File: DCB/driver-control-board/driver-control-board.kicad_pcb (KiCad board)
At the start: 2 copper layers, 92.7 x 59.2 mm, 33 parts, among them J1 Conn_01x05, J2 Conn_01x14, J3 Conn_01x08, J4 Conn_01x23, U1 STM32F413CGUx, U2 LD1117S33TR_SOT223, U3 R-78B5.0-2.0, U4 MCP2551-I-SN, Y1 Crystal

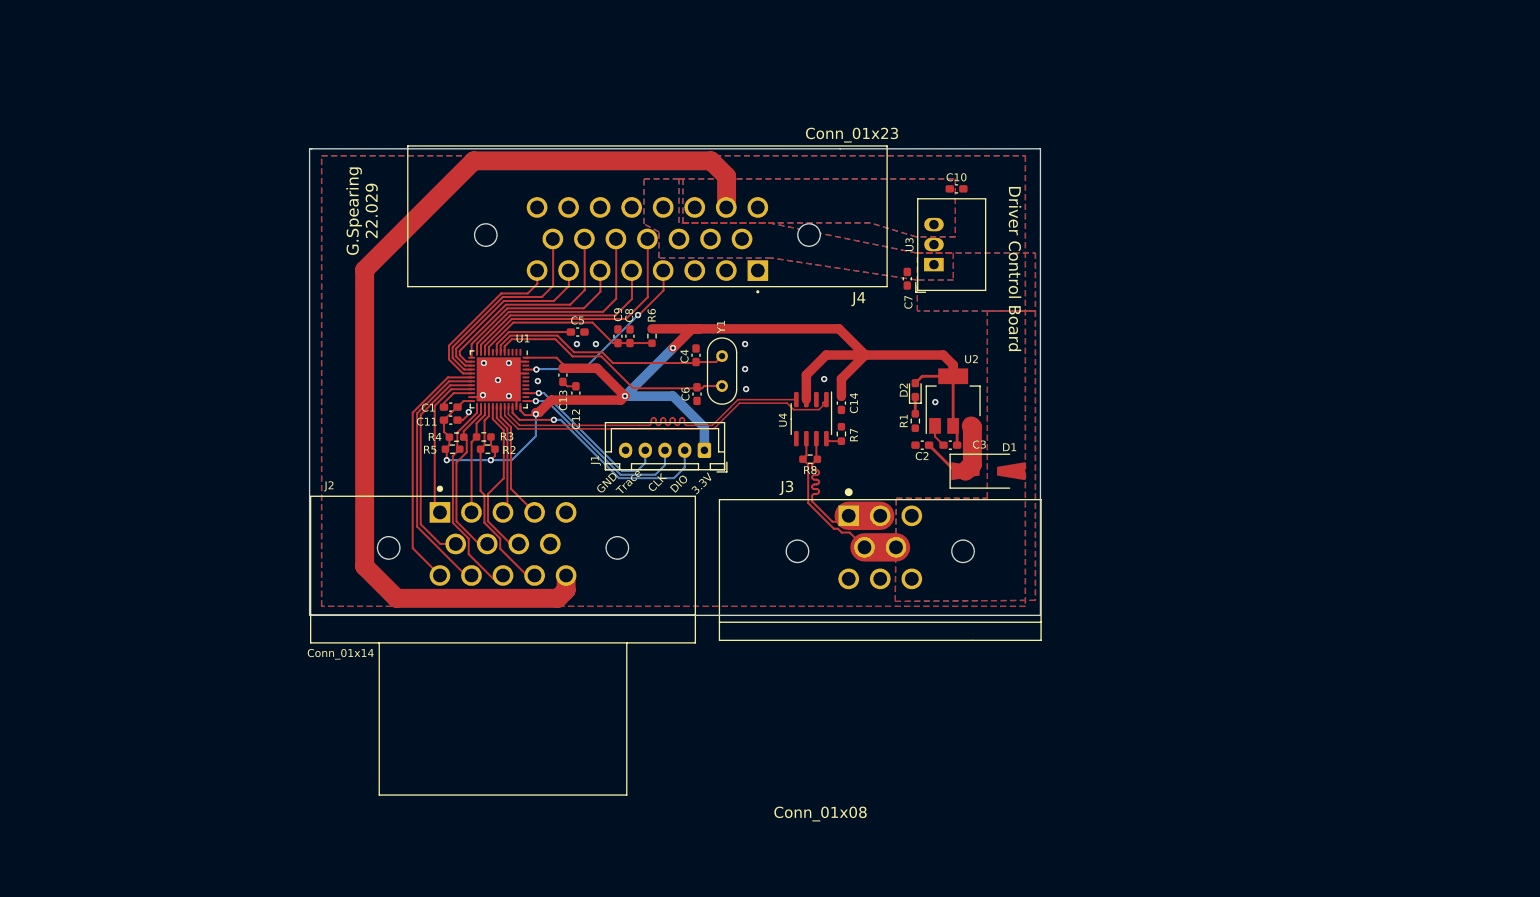
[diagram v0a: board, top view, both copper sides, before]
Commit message: working on layout
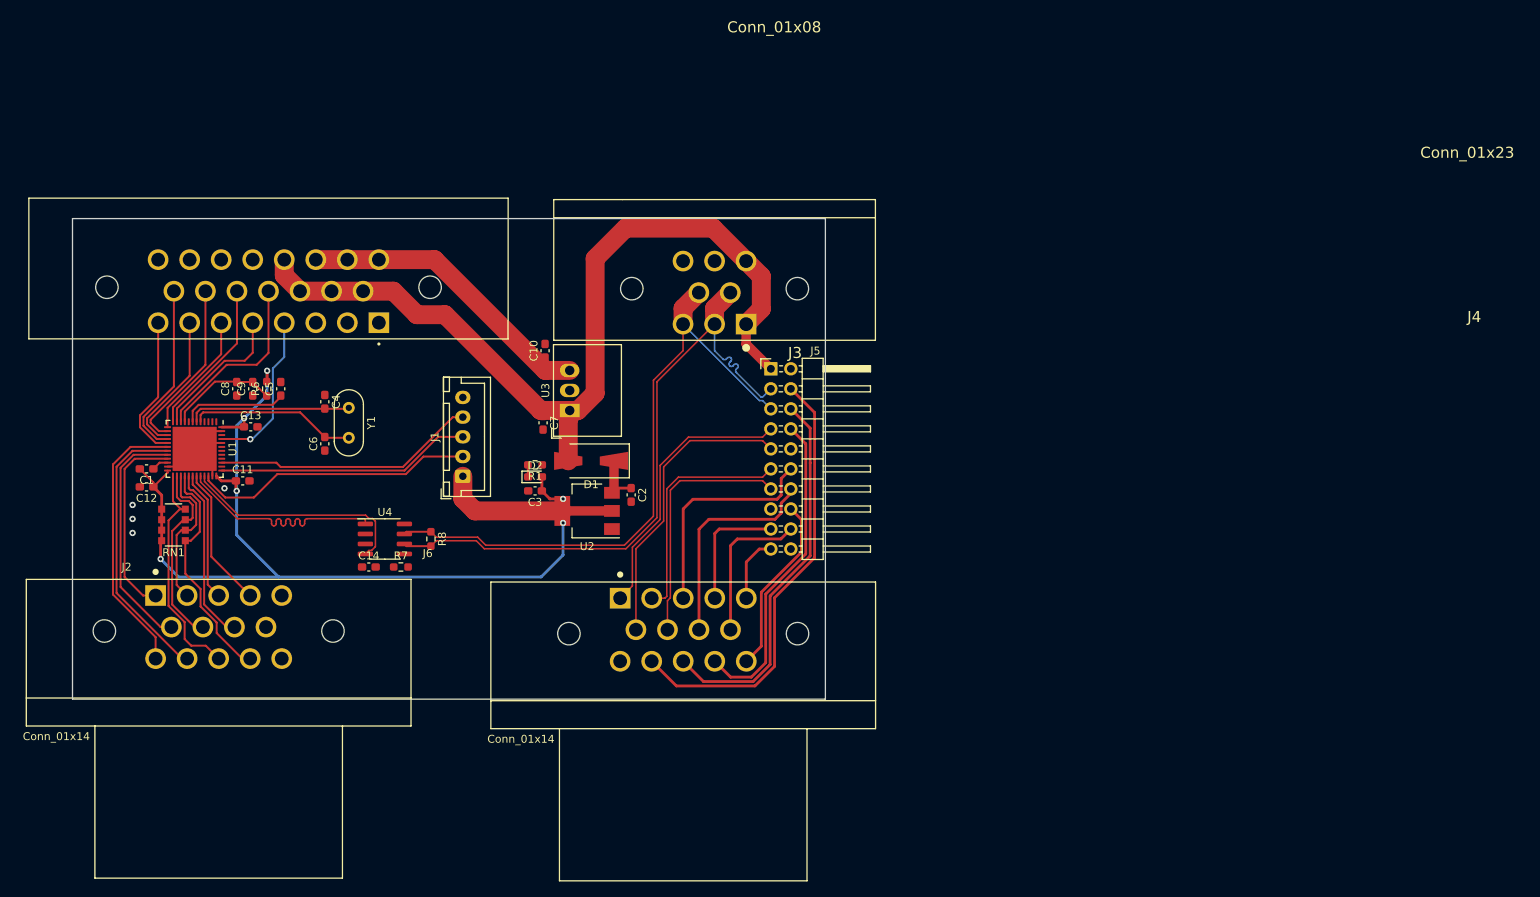
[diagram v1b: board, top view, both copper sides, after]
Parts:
- removed R2, R3, R4, R5: 10k, Resistor_SMD:R_0603_1608Metric_Pad0.98x0.95mm_HandSolder
- added J5: Conn_02x10_Counter_Clockwise, Connector_PinHeader_2.54mm:PinHeader_2x10_P2.54mm_Horizontal, F.Cu at (152.1, 95.3)
- added J6: Conn_01x14, AERO_Footprints:TE_1-776266-1_14pin_Horizontal, F.Cu at (141.0, 128.4)
- added RN1: R_Pack04, Resistor_SMD:R_Array_Convex_4x1206, F.Cu at (76.3, 115.1)
- moved C14 63.4 mm to (101.1, 120.4), turned to 0 degrees
- moved R7 58.4 mm to (105.2, 120.4), turned to 0 degrees
- moved U4 56.2 mm to (103.1, 116.8), turned to 0 degrees
- moved C10 56.1 mm to (123.4, 93.0), turned to 90 degrees
- moved C12 55.7 mm to (72.9, 110.2), turned to 180 degrees
- moved C3 53.0 mm to (122.2, 110.7)
- moved D1 50.4 mm to (129.3, 106.9), turned to 180 degrees
- moved C8 50.3 mm to (84.3, 97.8), turned to 90 degrees
- moved U3 49.8 mm to (126.6, 100.5)
- moved C7 49.7 mm to (123.2, 102.1)
- moved D2 49.5 mm to (122.2, 109.0), turned to 0 degrees
- moved R6 49.3 mm to (88.1, 97.8)
- moved R8 49.2 mm to (109.0, 116.8), turned to -90 degrees
- moved R1 48.6 mm to (122.2, 107.4), turned to 180 degrees
- moved J4 48.5 mm to (102.4, 89.4)
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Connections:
- J3 pad 1: /CAN_P -> +12V
- J3 pad 2: /CAN_P -> /CAN_N
- J3 pad 3: +12V -> /CAN_P
- J3 pad 5: /CAN_N -> /CAN_P
- J3 pad 6: GND -> +12V
- J3 pad 8: +12V -> GND
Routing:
- net +12V: track 0.00 -> 112.0 mm
- net +5V: track 123.6 -> 38.0 mm
- net /CAN_N: track 22.1 -> 82.4 mm
- net /CAN_P: track 22.8 -> 80.3 mm
- net /12V_OUT: track 0.00 -> 56.5 mm
- net /5V_OUT: track 0.00 -> 48.5 mm
- net /Heater: track 0.00 -> 40.6 mm
- net /DISP-: track 0.00 -> 37.5 mm
- net /DISP+: track 0.00 -> 34.9 mm
- net /USB_D-: track 0.00 -> 31.5 mm
- net /USB_D+: track 0.00 -> 29.9 mm
- net /USB_GND: track 0.00 -> 28.3 mm
- net /USB_PWR: track 0.00 -> 27.6 mm
- net /CURRENT_GND: track 0.00 -> 22.8 mm
- net /CURRENT_2: track 0.00 -> 19.2 mm
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- removed copper zone on B.Cu, net +12V
- removed copper zone on F.Cu, net +12V
- removed copper zone on B.Cu, net +5V
- removed copper zone on F.Cu, net +5V
- removed copper zone on B.Cu, net GND
- removed copper zone on F.Cu, net GND
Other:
- board size 92.7 x 59.2 mm -> 95.5 x 61 mm
- board text removed: "3.3V"
- board text removed: "CLK"
- board text removed: "DIO"
- board text removed: "Driver Control Board"
- board text removed: "G.Spearing 22.029"
- board text removed: "GND"
- board text removed: "Trace"
